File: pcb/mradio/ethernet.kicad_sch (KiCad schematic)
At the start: 30 parts, among them J301 JX0026D21BNL, Q301 DN2540N3-G, U301 DP83825I, Y301 DSC1525JL2A-25M00000T

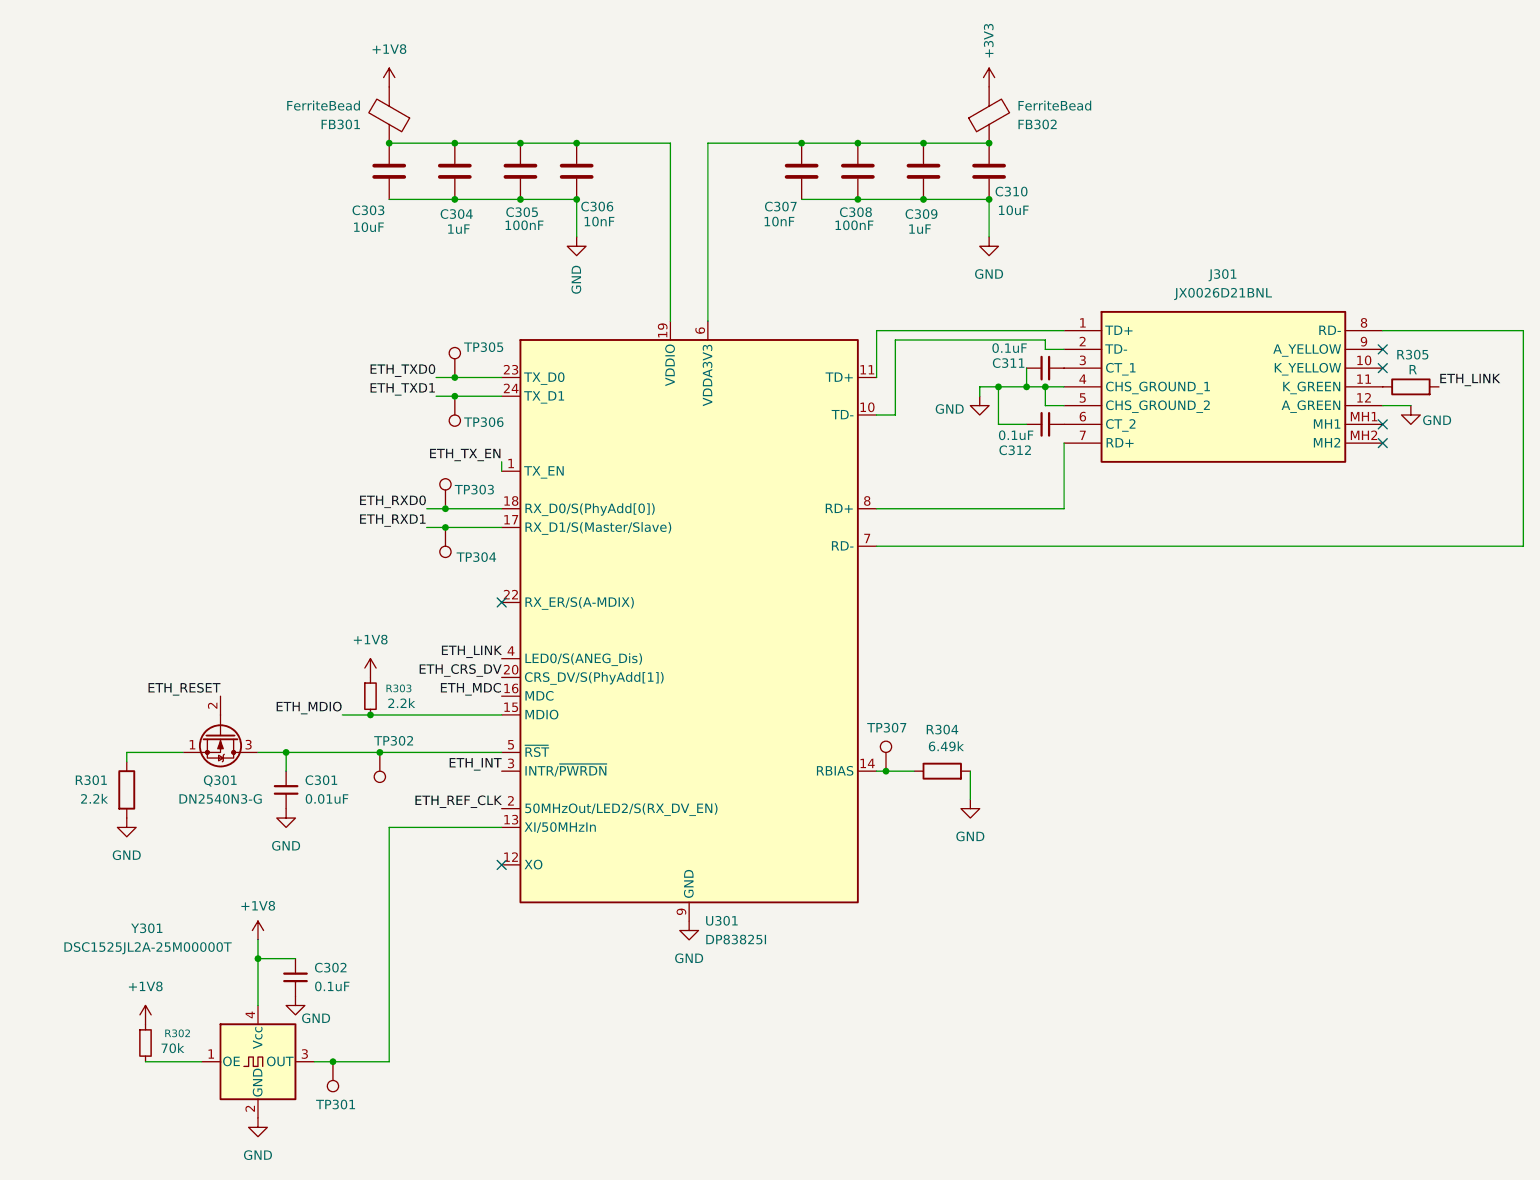
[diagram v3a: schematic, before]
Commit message: ethernet erc
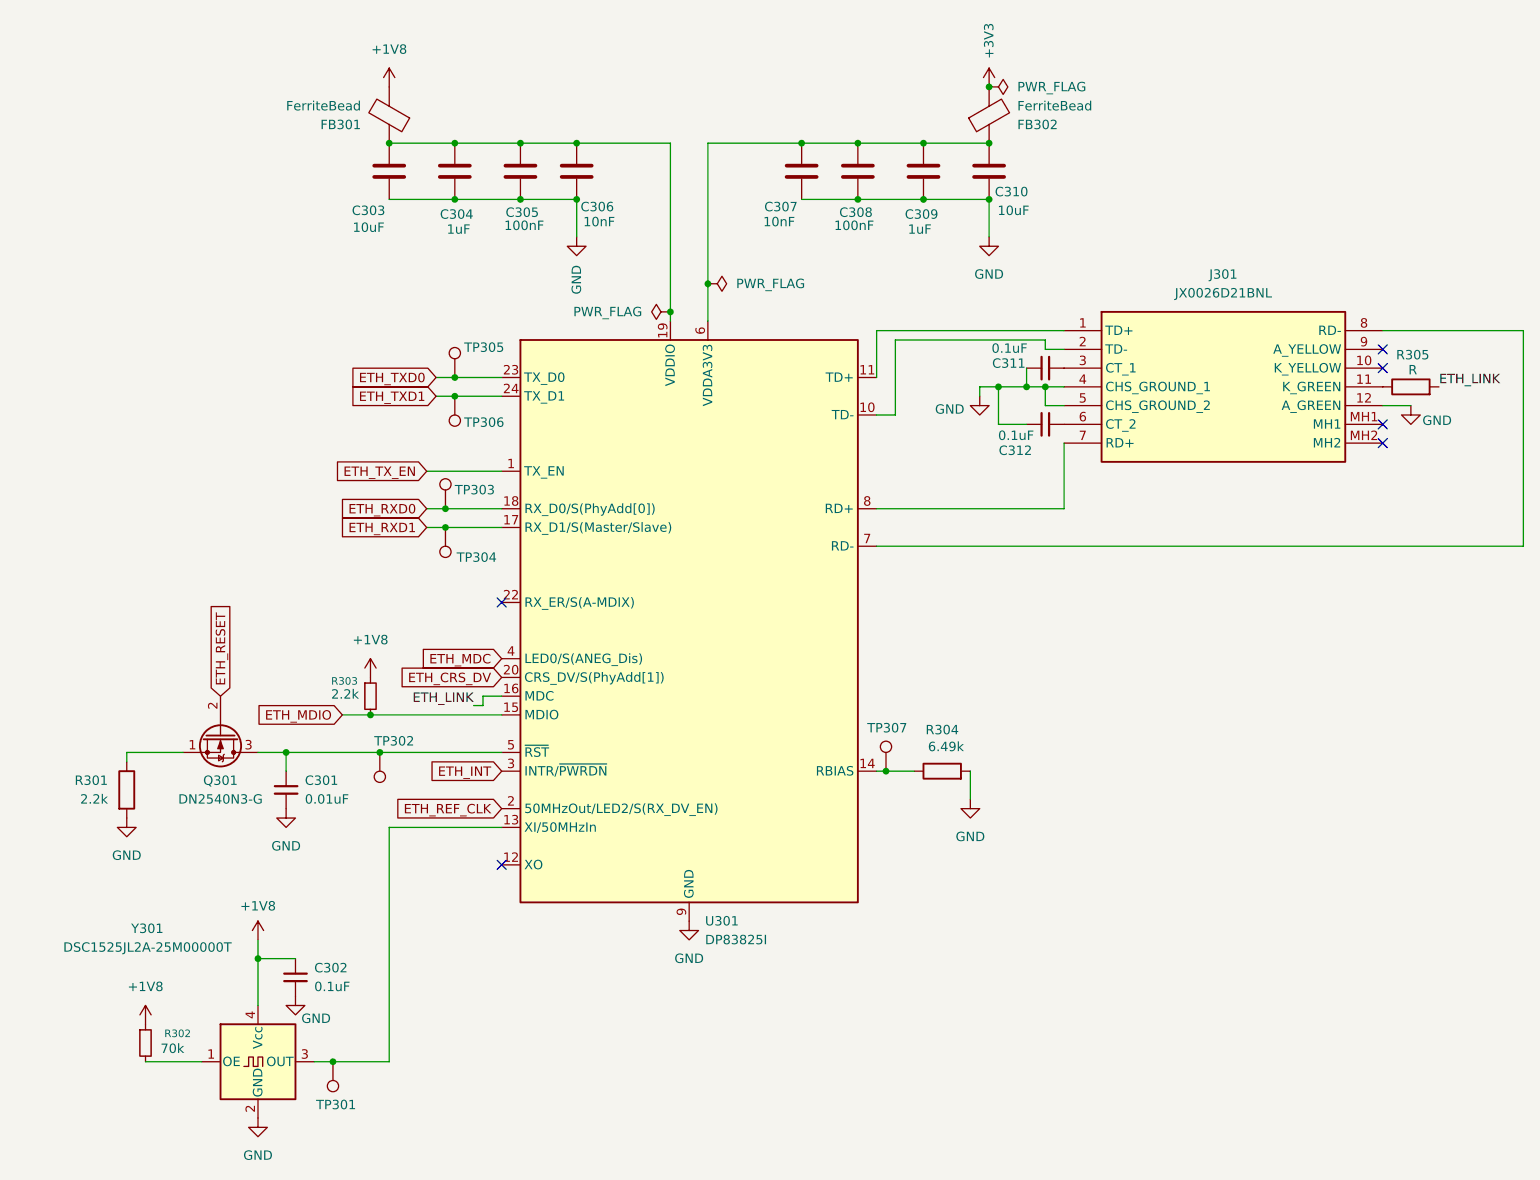
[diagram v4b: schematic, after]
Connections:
- net ETH_LINK: now also U301.16 (MDC); no longer U301.4 (LED0/S(ANEG_Dis))
- net ETH_MDC: now also U301.4 (LED0/S(ANEG_Dis)); no longer U301.16 (MDC)
